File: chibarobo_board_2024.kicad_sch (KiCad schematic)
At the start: 0 parts

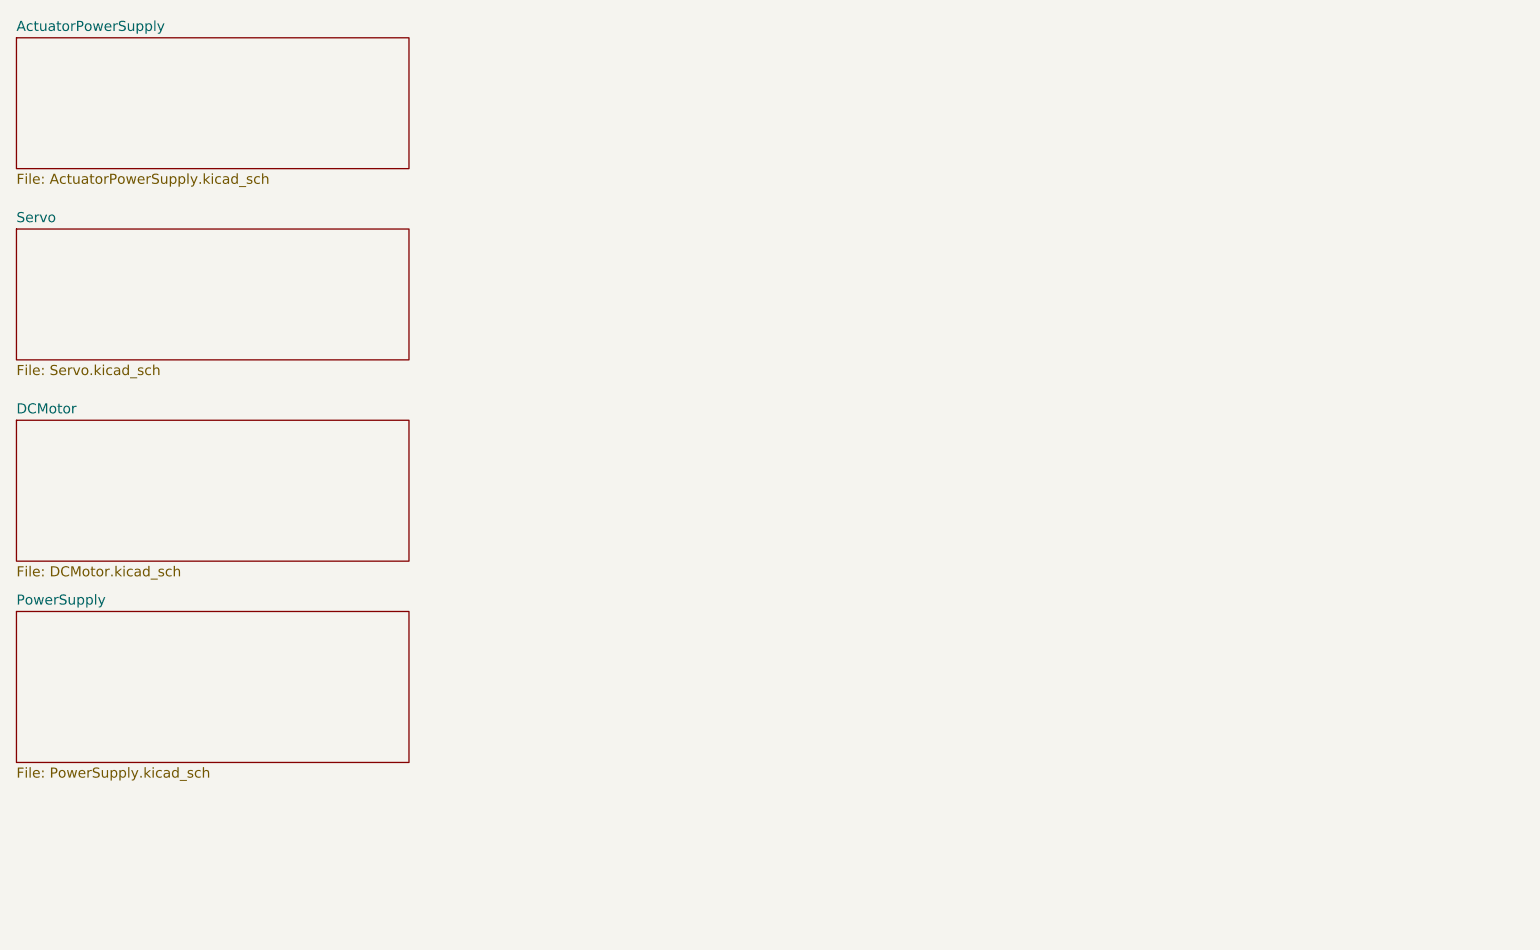
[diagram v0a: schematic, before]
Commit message: CircuitComplete
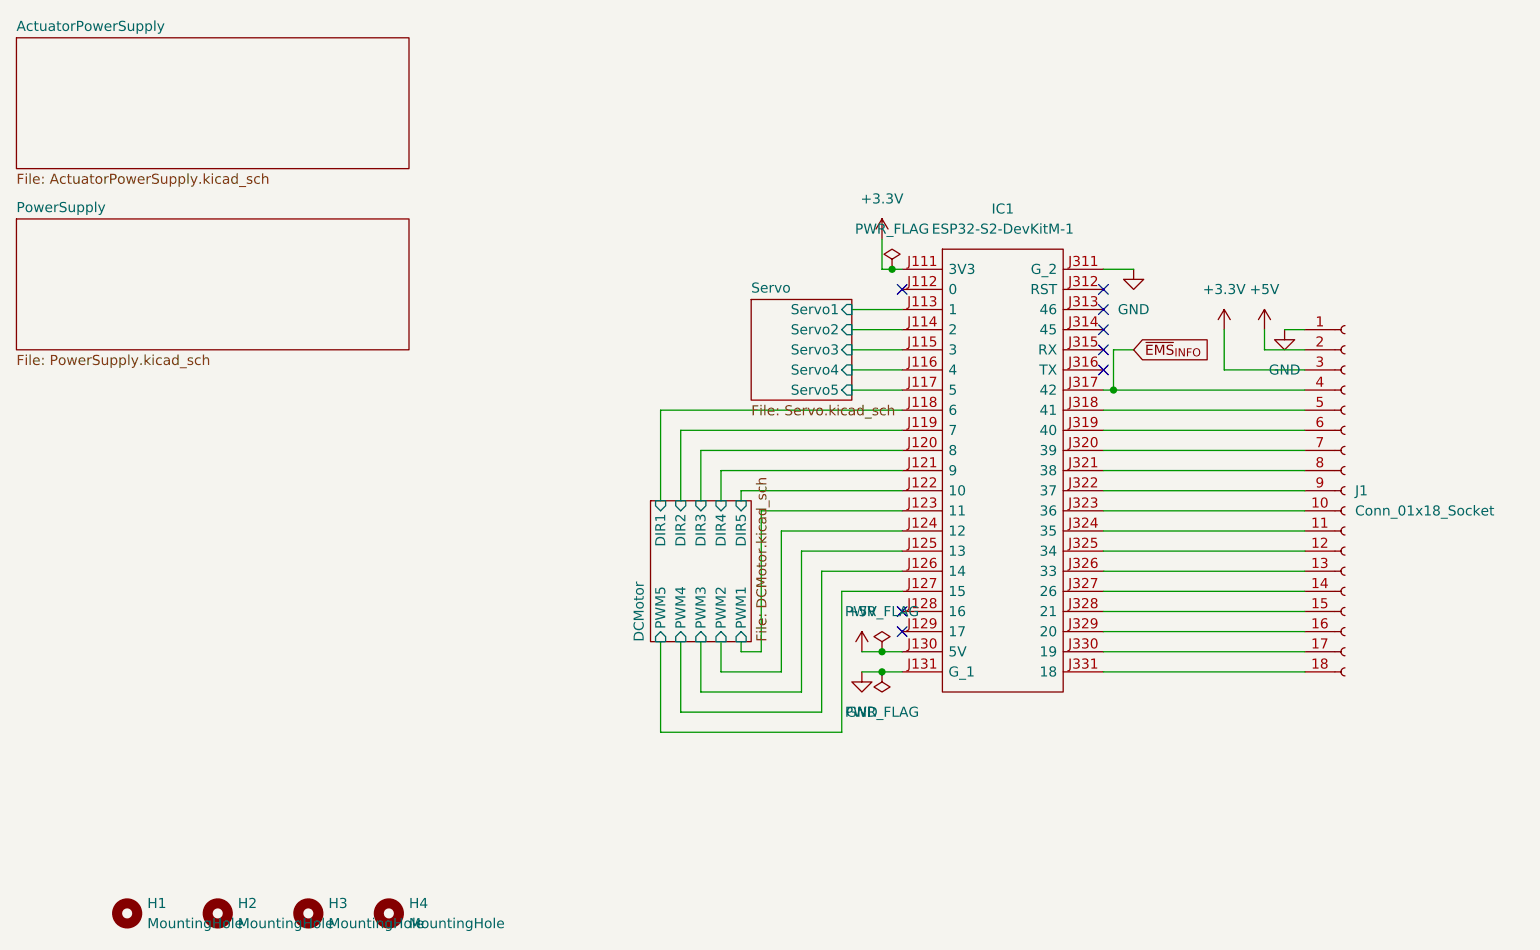
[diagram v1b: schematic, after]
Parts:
- added H1, H2, H3, H4: MountingHole, MountingHole:MountingHole_3.2mm_M3, symbol Mechanical:MountingHole
- added IC1: ESP32-S2-DevKitM-1, original:ESP32S2DevKitM1, symbol SamacSys_Parts:ESP32-S2-DevKitM-1
- added J1: Conn_01x18_Socket, Connector_PinHeader_2.54mm:PinHeader_2x09_P2.54mm_Vertical, symbol Connector:Conn_01x18_Socket
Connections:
- new net: IC1.J318 (41), J1.5 (Pin_5)
- new net: IC1.J319 (40), J1.6 (Pin_6)
- new net: IC1.J320 (39), J1.7 (Pin_7)
- new net: IC1.J321 (38), J1.8 (Pin_8)
- new net: IC1.J322 (37), J1.9 (Pin_9)
- new net: IC1.J323 (36), J1.10 (Pin_10)
- new net: IC1.J324 (35), J1.11 (Pin_11)
- new net: IC1.J325 (34), J1.12 (Pin_12)
- new net: IC1.J326 (33), J1.13 (Pin_13)
- new net: IC1.J327 (26), J1.14 (Pin_14)
- new net: IC1.J328 (21), J1.15 (Pin_15)
- new net: IC1.J329 (20), J1.16 (Pin_16)
- new net: IC1.J330 (19), J1.17 (Pin_17)
- new net: IC1.J331 (18), J1.18 (Pin_18)
- new net +3.3V: IC1.J111 (3V3), J1.3 (Pin_3)
- new net +5V: IC1.J130 (5V), J1.2 (Pin_2)
- new net DCMotor/DIR1: IC1.J118 (6)
- new net DCMotor/DIR2: IC1.J119 (7)
- new net DCMotor/DIR3: IC1.J120 (8)
- new net DCMotor/DIR4: IC1.J121 (9)
- new net DCMotor/DIR5: IC1.J122 (10)
- new net DCMotor/PWM1: IC1.J123 (11)
- new net DCMotor/PWM2: IC1.J124 (12)
- new net DCMotor/PWM3: IC1.J125 (13)
- new net DCMotor/PWM4: IC1.J126 (14)
- new net DCMotor/PWM5: IC1.J127 (15)
- new net GND: IC1.J131 (G_1), IC1.J311 (G_2), J1.1 (Pin_1)
- new net Servo/Servo1: IC1.J113 (1)
- new net Servo/Servo2: IC1.J114 (2)
- new net Servo/Servo3: IC1.J115 (3)
- new net Servo/Servo4: IC1.J116 (4)
- new net Servo/Servo5: IC1.J117 (5)
- new net ~{EMS}_{INFO}: IC1.J317 (42), J1.4 (Pin_4)
- no-connect marks 0 -> 8
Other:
- sheet DCMotor ports: added DIR1, DIR2, DIR3, DIR4, DIR5, PWM1, PWM2, PWM3, PWM4, PWM5; removed none
- sheet Servo ports: added Servo1, Servo2, Servo3, Servo4, Servo5; removed none
